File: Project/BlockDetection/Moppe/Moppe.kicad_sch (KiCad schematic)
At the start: 51 parts, among them J1 Conn_01x02_Pin, J2 Conn_01x02_Pin, J3 Conn_01x02_Pin, J4 Conn_01x02_Pin, J5 Conn_01x02_Pin, J6 Conn_01x02_Pin, J7 Amphenol RJHSE5380, J8 Conn_01x02_Pin, J9 Conn_01x03_Socket, Q1 BC856, Q2 BC856 or BC557, Q3 BC856 or BC557, Q4 BC856 or BC557, Q5 BC557, Q6 BC547, U1 PC847, U2 PC817, U4 TLP620

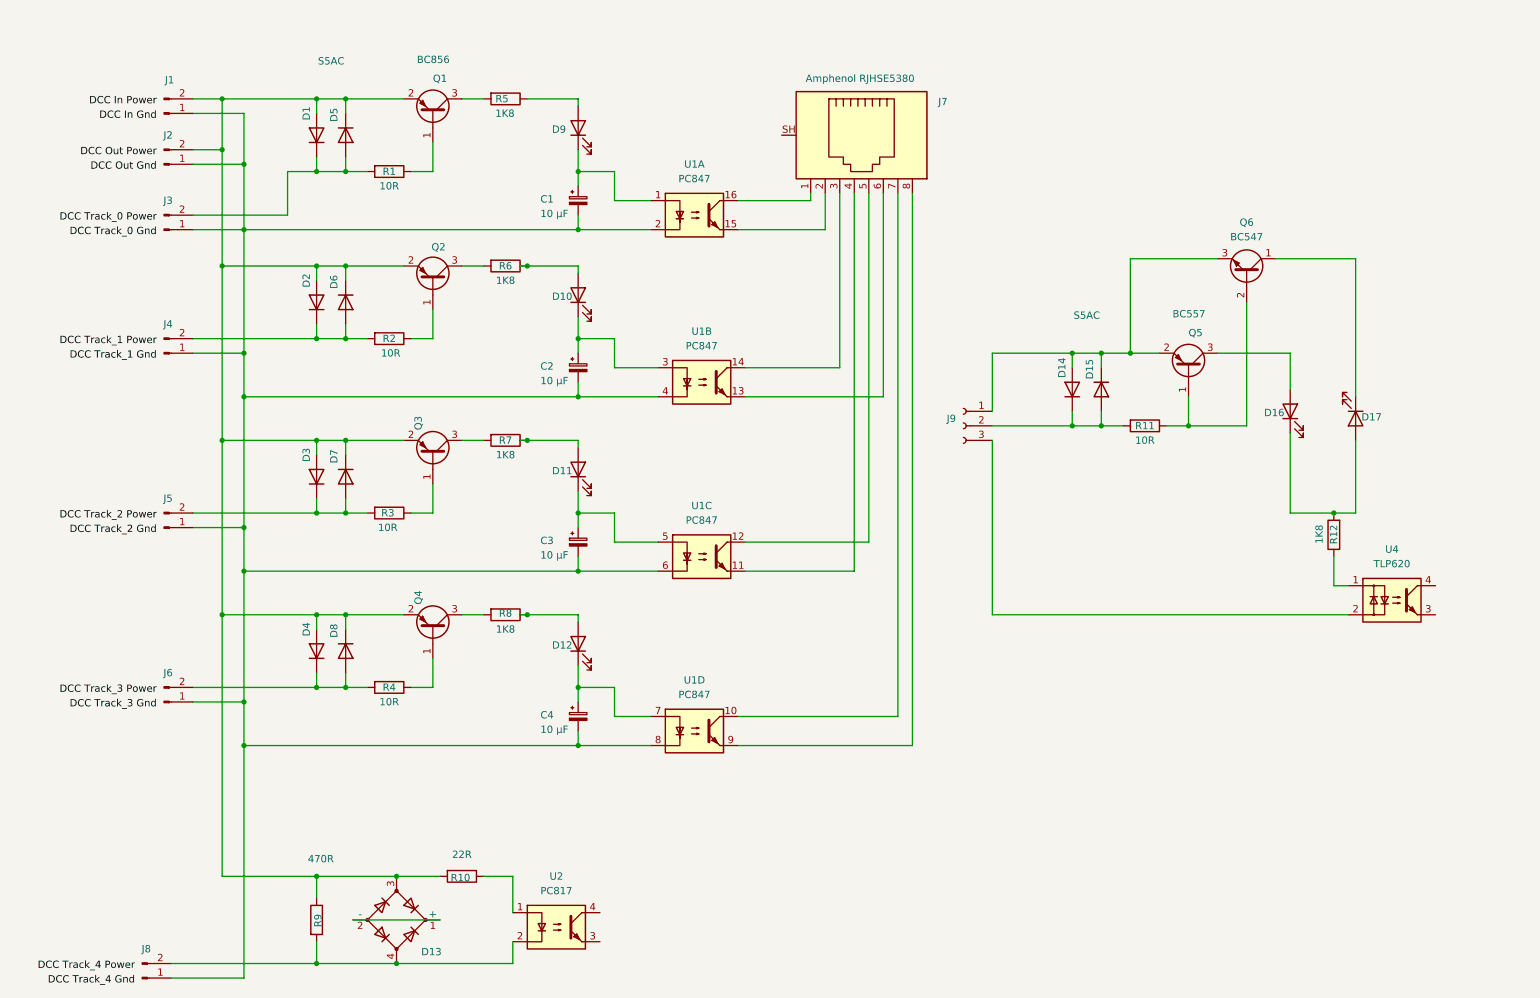
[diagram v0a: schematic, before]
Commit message: efter test
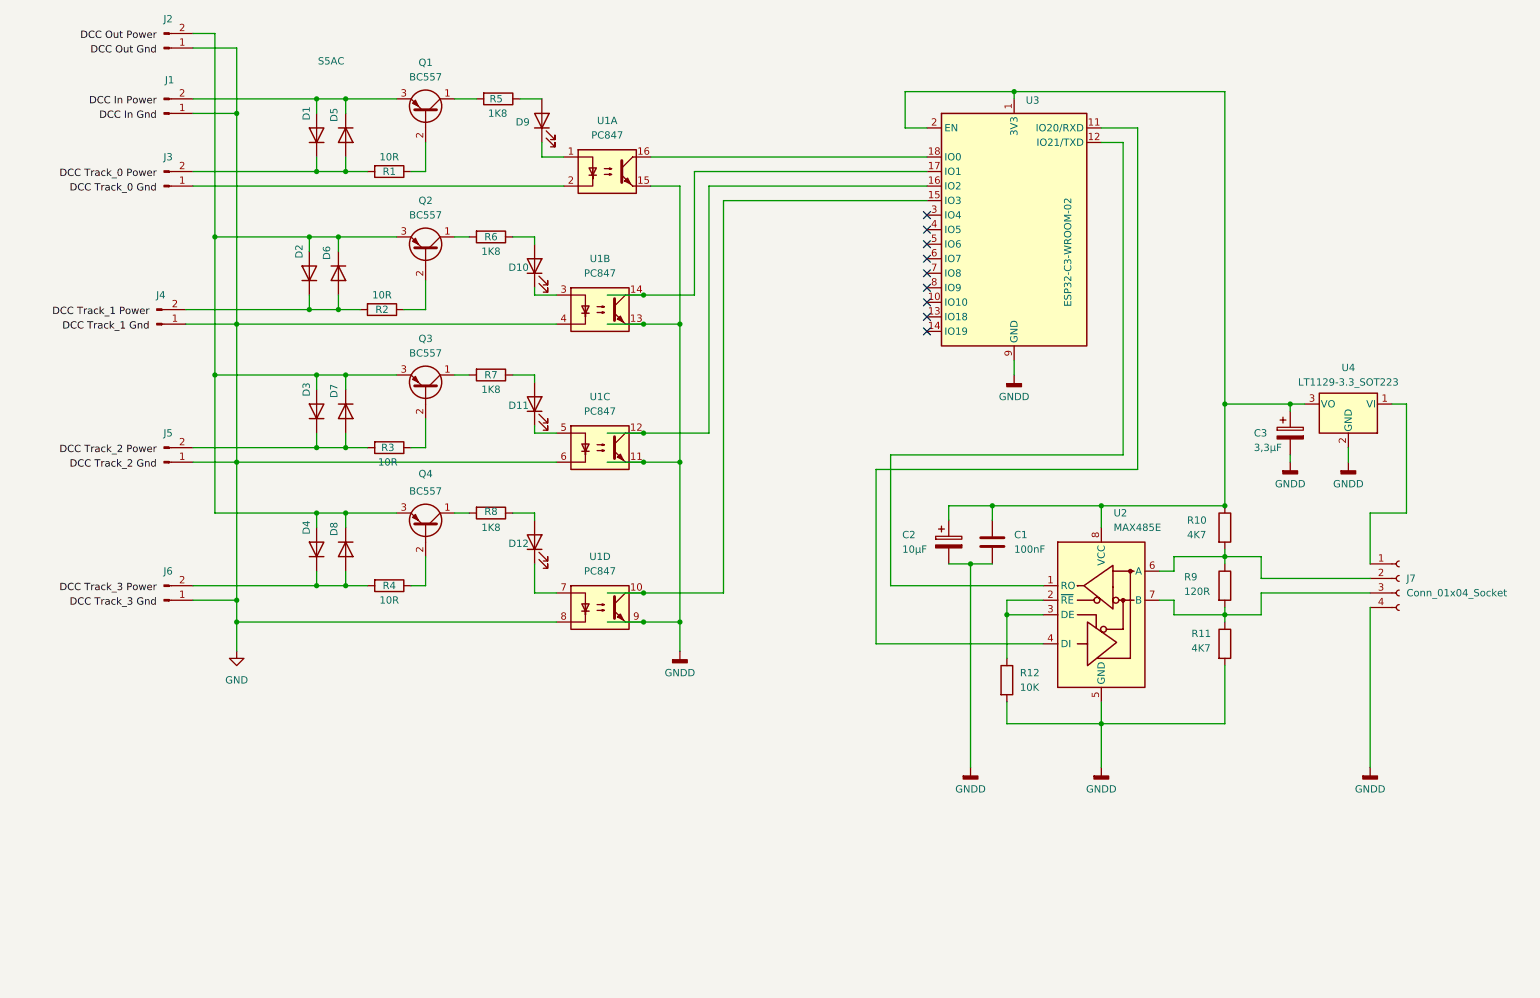
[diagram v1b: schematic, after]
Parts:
- removed C1, C2, C3, C4: 10 µF, symbol Device:C_Polarized_Small
- removed D13: D_Bridge_+-AA, Module:Pololu_Breakout-16_15.2x20.3mm, symbol Device:D_Bridge_+-AA
- removed D14: S5AC, Diode_THT:D_DO-201AD_P15.24mm_Horizontal, symbol Diode:1N5400
- removed D15: 1N5400, Diode_THT:D_DO-201AD_P15.24mm_Horizontal, symbol Diode:1N5400
- removed D16, D17: IR26-21C_L110_TR8, LED_SMD:LED_1206_3216Metric, symbol LED:IR26-21C_L110_TR8
- removed J7: Amphenol RJHSE5380, Connector_RJ:RJ45_Amphenol_RJHSE5380, symbol Connector:RJ45_Shielded
- removed J8: Conn_01x02_Pin, Connector:Tag-Connect_TC2030-IDC-FP_2x03_P1.27mm_Vertical, symbol Connector:Conn_01x02_Pin
- removed J9: Conn_01x03_Socket, Package_TO_SOT_THT:TO-92_Inline, symbol Connector:Conn_01x03_Socket
- removed Q1: BC856, Package_TO_SOT_SMD:SOT-23, symbol Transistor_BJT:BC856
- removed Q2, Q3, Q4: BC856 or BC557, Package_TO_SOT_SMD:SOT-23, symbol Transistor_BJT:BC856
- removed Q5: BC557, Package_TO_SOT_SMD:SOT-23, symbol Transistor_BJT:BC856
- removed Q6: BC547, Package_TO_SOT_THT:TO-92_Inline, symbol Transistor_BJT:BC547
- removed U2: PC817, Package_DIP:DIP-4_W7.62mm, symbol Isolator:PC817
- removed U4: TLP620, Package_SO:SOP-4_4.4x2.6mm_P1.27mm, symbol Isolator:TLP290
- added C1: 100nF, symbol Device:C
- added C2: 10µF, Package_QFP:LQFP-100_14x14mm_P0.5mm, symbol Device:C_Polarized
- added C3: 3,3µF, Package_QFP:LQFP-100_14x14mm_P0.5mm, symbol Device:C_Polarized
- added J7: Conn_01x04_Socket, Connector:Tag-Connect_TC2030-IDC-NL_2x03_P1.27mm_Vertical, symbol Connector:Conn_01x04_Socket
- added Q1, Q2, Q3, Q4: BC557, Package_TO_SOT_THT:TO-92_Inline, symbol Transistor_BJT:BC557
- added U2: MAX485E, Package_SO:SOIC-8_3.9x4.9mm_P1.27mm, symbol Interface_UART:MAX485E
- added U3: ESP32-C3-WROOM-02, RF_Module:ESP32-C3-WROOM-02, symbol RF_Module:ESP32-C3-WROOM-02
- added U4: LT1129-3.3_SOT223, Package_TO_SOT_SMD:SOT-223-3_TabPin2, symbol Regulator_Linear:LT1129-3.3_SOT223
- R10: value 22R -> 4K7; footprint (none) -> Inductor_THT:L_CommonMode_PulseElectronics_PH9455x105NL_1
- R11: value 10R -> 4K7; footprint (none) -> Inductor_THT:L_CommonMode_PulseElectronics_PH9455x105NL_1
- R12: value 1K8 -> 10K; footprint (none) -> Inductor_THT:L_CommonMode_PulseElectronics_PH9455x105NL_1
- R9: value 470R -> 120R; footprint (none) -> Inductor_THT:L_CommonMode_PulseElectronics_PH9455x105NL_1
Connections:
- net at R11.1: now also R9.2, J7.3 (Pin_3), U2.7 (B)
- net GND: now reaches J1.1 (Pin_1), J2.1 (Pin_1), J4.1 (Pin_1), J5.1 (Pin_1), J6.1 (Pin_1), U1.4, U1.6, U1.8
- net GND: no longer J3.1 (Pin_1), U1.2
- net GNDD: now reaches U1.15
- net GNDD: now also R11.2, R12.2, U1.11, U1.13, U1.9, C1.2, C2.2, C3.2, J7.4 (Pin_4), U2.5 (GND), U3.19 (GND), U3.9 (GND), U4.2 (GND)
- net at U1.16: now also U3.18 (IO0)
- net at D2.2 (A), D3.2 (A), D4.2 (A)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: now also Q2.3 (E), Q3.3 (E), Q4.3 (E); no longer D1.2 (A), D5.1 (K), J1.2 (Pin_2), R10.2, R9.1
- net at R12.1: now also U2.2 (~{RE}), U2.3 (DE)
- net at R5.2: now also Q1.1 (C)
- net at R6.2: now also Q2.1 (C)
- net at R2.1: now also Q2.2 (B)
- net at U1.12: now also U3.16 (IO2)
- net at R10.1: now also C1.1, C2.1, C3.1, U2.8 (VCC), U3.1 (3V3), U3.2 (EN), U4.3 (VO)
- net at R7.2: now also Q3.1 (C)
- net at U1.14: now also U3.17 (IO1)
- net at R3.1: now also Q3.2 (B)
- net at R4.1: now also Q4.2 (B)
- net at U1.10: now also U3.15 (IO3)
- net at R8.2: now also Q4.1 (C)
- net at R1.1: now also Q1.2 (B)
- new net: J3.1 (Pin_1), U1.2
- new net: U2.1 (RO), U3.12 (IO21/TXD)
- new net: U2.4 (DI), U3.11 (IO20/RXD)
- new net: J7.2 (Pin_2), R10.2, R9.1, U2.6 (A)
- new net: D1.2 (A), D5.1 (K), J1.2 (Pin_2), Q1.3 (E)
- new net: J7.1 (Pin_1), U4.1 (VI)
- no-connect marks 0 -> 9
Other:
- moved on the sheet: D10, D11, D12, D2, D3, D4, D6, D7, D8, D9, J2, J3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
